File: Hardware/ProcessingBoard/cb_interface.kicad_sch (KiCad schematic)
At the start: 1 part, among them J1 Conn_01x30_MountingPin

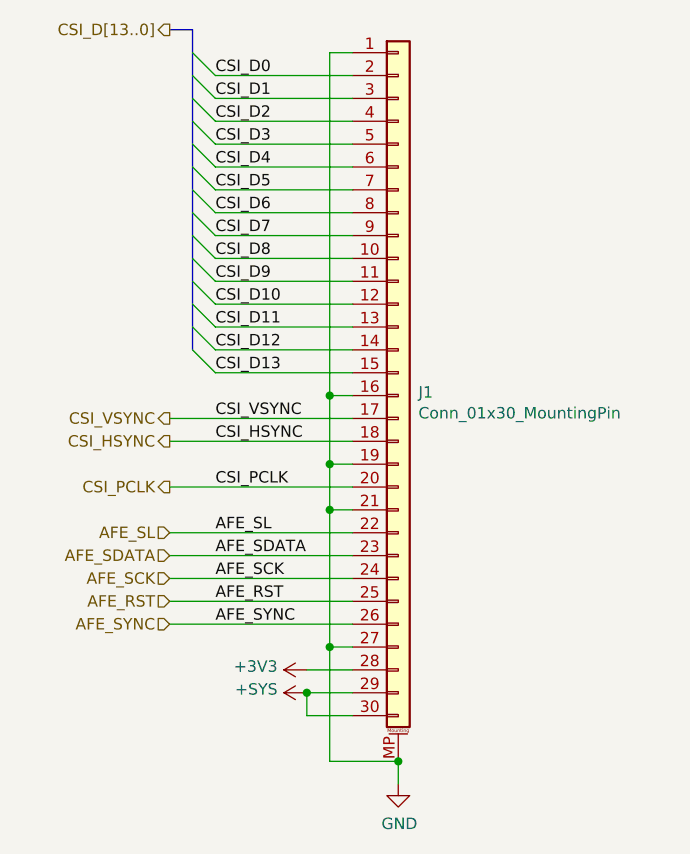
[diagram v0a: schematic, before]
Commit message: Bug fixes and changes for PB r0p2
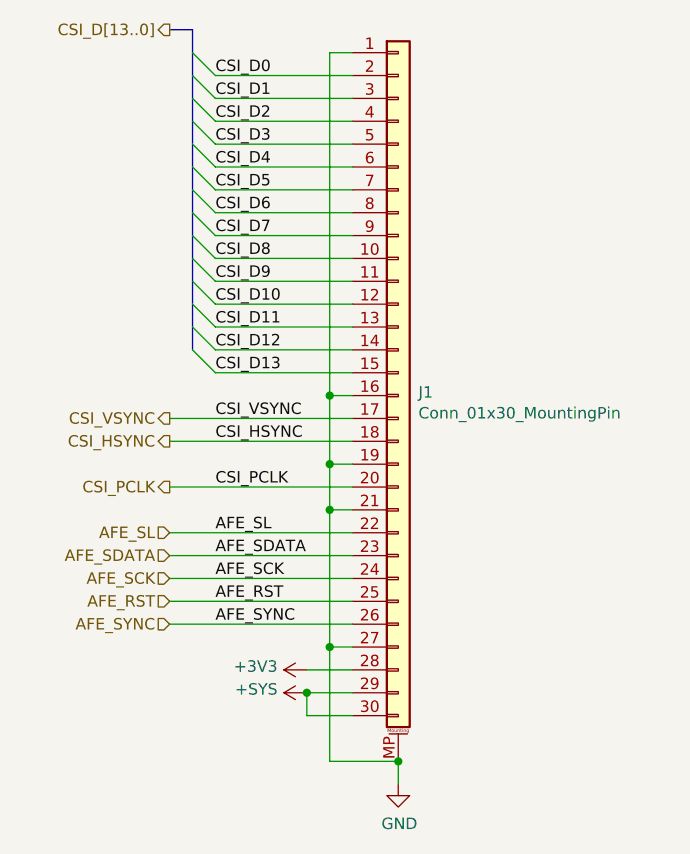
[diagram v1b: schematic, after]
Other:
- company: (none) -> Wenting
- title: (none) -> SitinaNe
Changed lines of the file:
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@@
 (kicad_sch (version 20210126) (generator eeschema)
   (paper "A4")
+  (title_block
+    (title "SitinaNe")
+    (rev "R0.2")
+    (company "Wenting")
+  )
   (junction (at 152.4 134.62) (diameter 0.9144) (color 0 0 0 0))
   (junction (at 154.94 101.6) (diameter 0.9144) (color 0 0 0 0))
@@
     (stroke (width 0) (type solid) (color 0 0 0 0))
   )
-  (bus (pts (xy 139.7 60.96) (xy 139.7 96.52))
-    (stroke (width 0) (type solid) (color 0 0 0 0))
-  )
+  (bus (pts (xy 139.7 60.96) (xy 139.7 63.5))
+    (stroke (width 0) (type solid) (color 0 0 0 0))
+  )
+  (bus (pts (xy 139.7 63.5) (xy 139.7 66.04))
+    (stroke (width 0) (type solid) (color 0 0 0 0))
+  )
+  (bus (pts (xy 139.7 66.04) (xy 139.7 68.58))
+    (stroke (width 0) (type solid) (color 0 0 0 0))
+  )
+  (bus (pts (xy 139.7 68.58) (xy 139.7 71.12))
+    (stroke (width 0) (type solid) (color 0 0 0 0))
+  )
+  (bus (pts (xy 139.7 71.12) (xy 139.7 73.66))
+    (stroke (width 0) (type solid) (color 0 0 0 0))
+  )
+  (bus (pts (xy 139.7 73.66) (xy 139.7 76.2))
+    (stroke (width 0) (type solid) (color 0 0 0 0))
+  )
+  (bus (pts (xy 139.7 76.2) (xy 139.7 78.74))
+    (stroke (width 0) (type solid) (color 0 0 0 0))
+  )
+  (bus (pts (xy 139.7 78.74) (xy 139.7 81.28))
+    (stroke (width 0) (type solid) (color 0 0 0 0))
+  )
+  (bus (pts (xy 139.7 81.28) (xy 139.7 83.82))
+    (stroke (width 0) (type solid) (color 0 0 0 0))
+  )
+  (bus (pts (xy 139.7 83.82) (xy 139.7 86.36))
+    (stroke (width 0) (type solid) (color 0 0 0 0))
+  )
+  (bus (pts (xy 139.7 86.36) (xy 139.7 88.9))
+    (stroke (width 0) (type solid) (color 0 0 0 0))
+  )
+  (bus (pts (xy 139.7 88.9) (xy 139.7 91.44))
+    (stroke (width 0) (type solid) (color 0 0 0 0))
+  )
+  (bus (pts (xy 139.7 91.44) (xy 139.7 93.98))
+    (stroke (width 0) (type solid) (color 0 0 0 0))
+  )
+  (bus (pts (xy 139.7 93.98) (xy 139.7 96.52))
+    (stroke (width 0) (type solid) (color 0 0 0 0))
+  )
